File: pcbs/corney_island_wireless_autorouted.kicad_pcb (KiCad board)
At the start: 2 copper layers, 114 x 91.6 mm, 84 parts

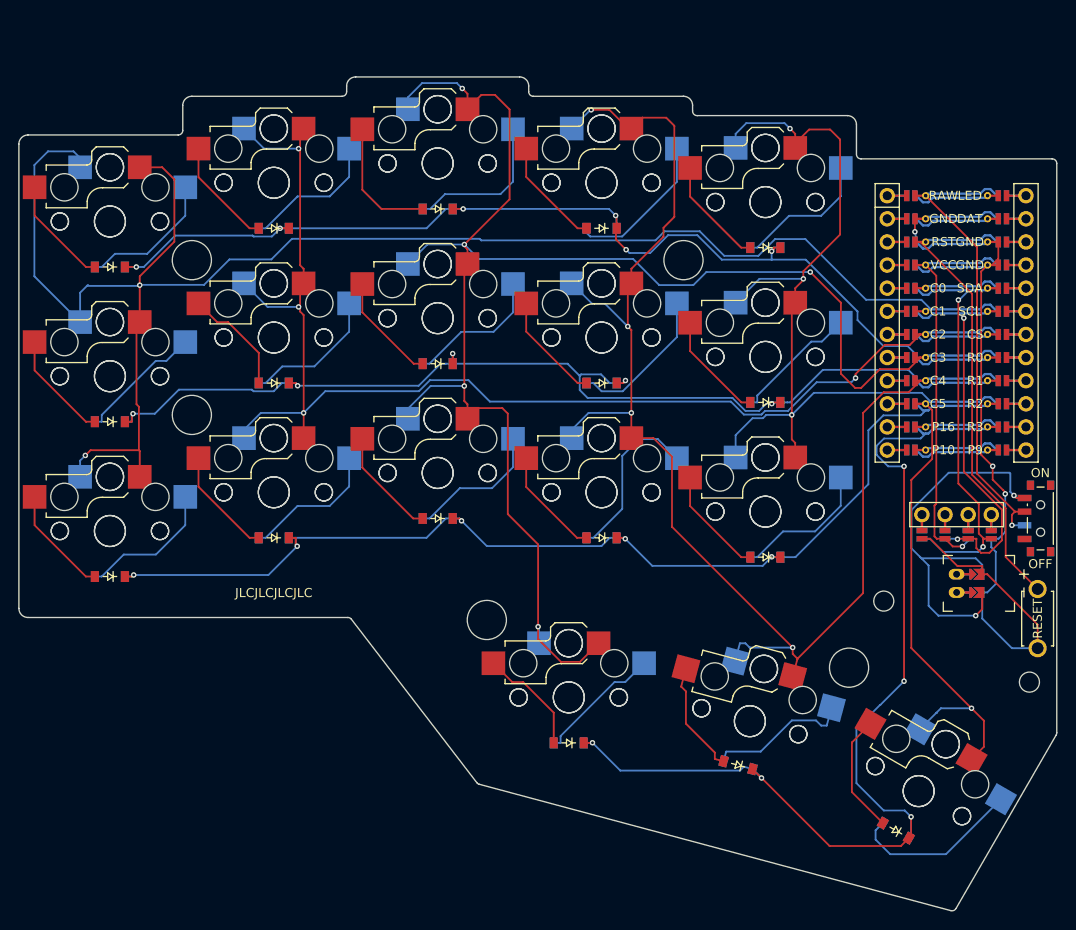
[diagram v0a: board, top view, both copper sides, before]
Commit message: staggero_change
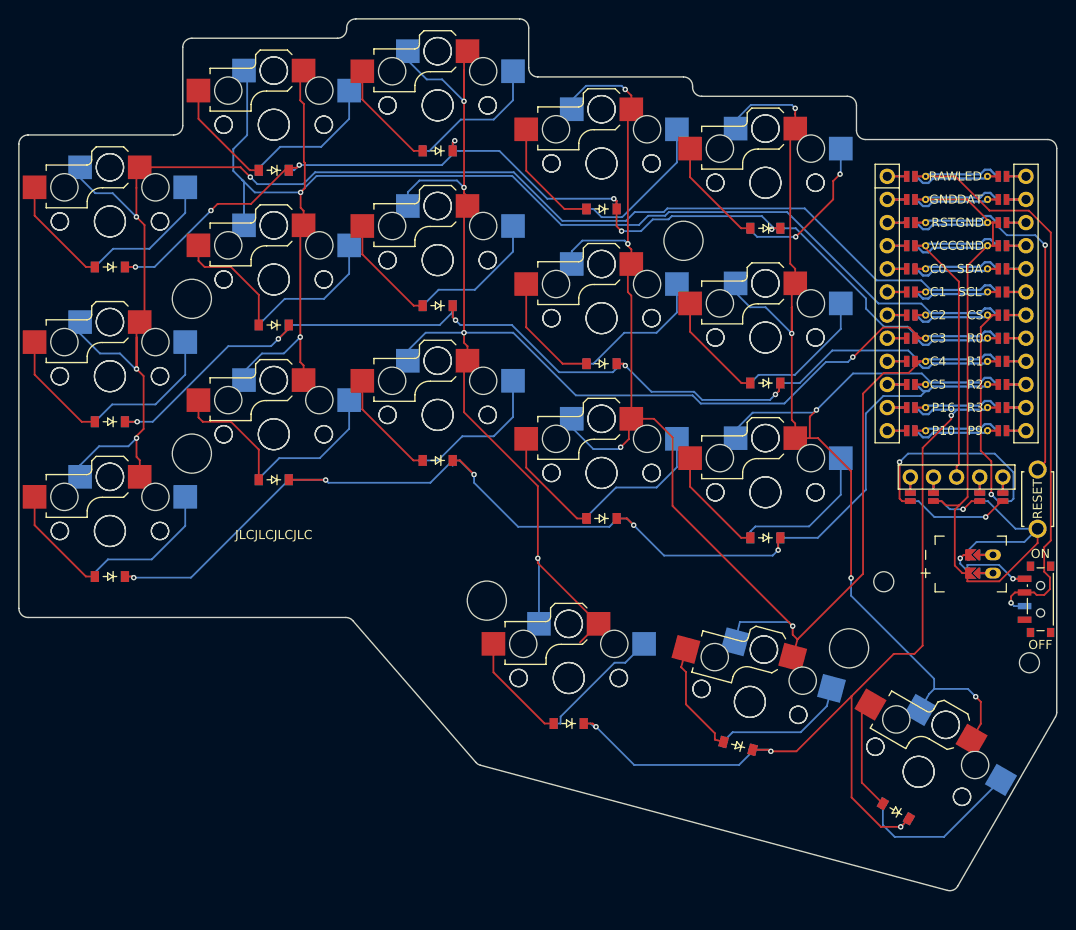
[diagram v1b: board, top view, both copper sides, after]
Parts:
- DISP1: footprint ceoloide:display_ssd1306 -> ceoloide:display_nice_view
- moved B1 13.1 mm to (201.9, 96.5)
- moved PWR1 8.88 mm to (202.2, 107.5)
- moved D22 6.38 mm to (118.0, 94.4)
- moved D23 6.38 mm to (118.0, 77.4)
- moved D24 6.38 mm to (118.0, 60.4)
- moved D25 6.38 mm to (136.0, 92.2)
- moved D26 6.38 mm to (136.0, 75.2)
- moved D27 6.38 mm to (136.0, 58.2)
- moved D4 6.38 mm to (118.0, 94.4)
- moved D5 6.38 mm to (118.0, 77.4)
- moved D6 6.38 mm to (118.0, 60.4)
- moved D7 6.38 mm to (136.0, 92.2)
- moved D8 6.38 mm to (136.0, 75.2)
- moved D9 6.38 mm to (136.0, 58.2)
- moved S22 6.38 mm to (118.0, 89.4)
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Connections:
- DISP1 pad 10: GND -> CS
- DISP1 pad 11: VCC -> GND
- DISP1 pad 12: SCL -> SCK
- DISP1 pad 13: SDA -> MOSI
- DISP1 pad 16: DISP1_3 -> DISP1_4
- DISP1 pad 17: DISP1_4 -> DISP1_5
- DISP1 pad 20: GND -> CS
- DISP1 pad 21: VCC -> GND
- DISP1 pad 22: SCL -> SCK
- DISP1 pad 23: SDA -> MOSI
- DISP1 pad 24: DISP1_4 -> DISP1_5
- DISP1 pad 25: DISP1_3 -> DISP1_4
- DISP1 pad 3: DISP1_3 -> VCC
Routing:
- net CS: track 9.96 -> 55.5 mm, vias 0 -> 2
- net SDA: track 48.3 -> 9.96 mm, vias 2 -> 0
- net SCL: track 44.9 -> 9.96 mm, vias 2 -> 0
- net BAT_P: track 45.8 -> 11.7 mm
- net RAW: track 52.8 -> 73.2 mm
- net C1: track 188.7 -> 171.7 mm, vias 2 -> 4
- net C2: track 141.8 -> 157.9 mm, vias 4 -> 2
- net R2: track 121.4 -> 134.6 mm
- net RST: track 53.4 -> 41.3 mm, vias 0 -> 1
- net MOSI: track 0.00 -> 11.6 mm, vias 0 -> 1
- net C3: track 184.7 -> 176.3 mm
- net VCC: track 45.5 -> 37.1 mm, vias 1 -> 0
- net R3: track 113.2 -> 106.8 mm, vias 5 -> 4
- net C5: track 150.5 -> 144.2 mm, vias 4 -> 5
- net SCK: track 0.00 -> 5.81 mm, vias 0 -> 1
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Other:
- board size 114 x 91.6 mm -> 114 x 95.8 mm
